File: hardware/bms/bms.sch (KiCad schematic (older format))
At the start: 199 parts, among them J1 Conn_01x08, J10 Conn_01x02, J11 Conn_01x02, J12 Conn_01x02, J13 Conn_01x10, J14 Conn_01x02, J15 Conn_01x02, J16 Cell Bypass, J2 Conn_01x04, J3 USB_B_Micro, J4 Conn_01x05, J5 Conn_01x04, J6 Conn_01x04, J7 Conn_01x03, J8 Conn_01x03, J9 Conn_01x02, M1 MountingHole, M2 MountingHole, M3 MountingHole, M4 MountingHole, M5 MountingHole, M6 MountingHole, Q1 BC817, Q10 ZXMP4A16G, Q11 IRF540N, Q12 IRF540N, Q13 BSS138, Q14 IRF540N, Q15 BSS138, Q16 BSS138, Q2 ZXMP4A16G, Q3 BSS138, Q4 BS170, Q5 IRF9540N, Q6 BC847, Q7 IRF9540N, Q8 BSS138, Q9 ZXMP4A16G, SW1 SW_DIP_x03, U1 USBLC6-2SC6, U2 STM32F042C6Tx, U3 TPS560430x3F, U4 TCAN334, U5 MAX485E, U6 LM5164DDAR, U7 LSI94202, Y1 8MHz

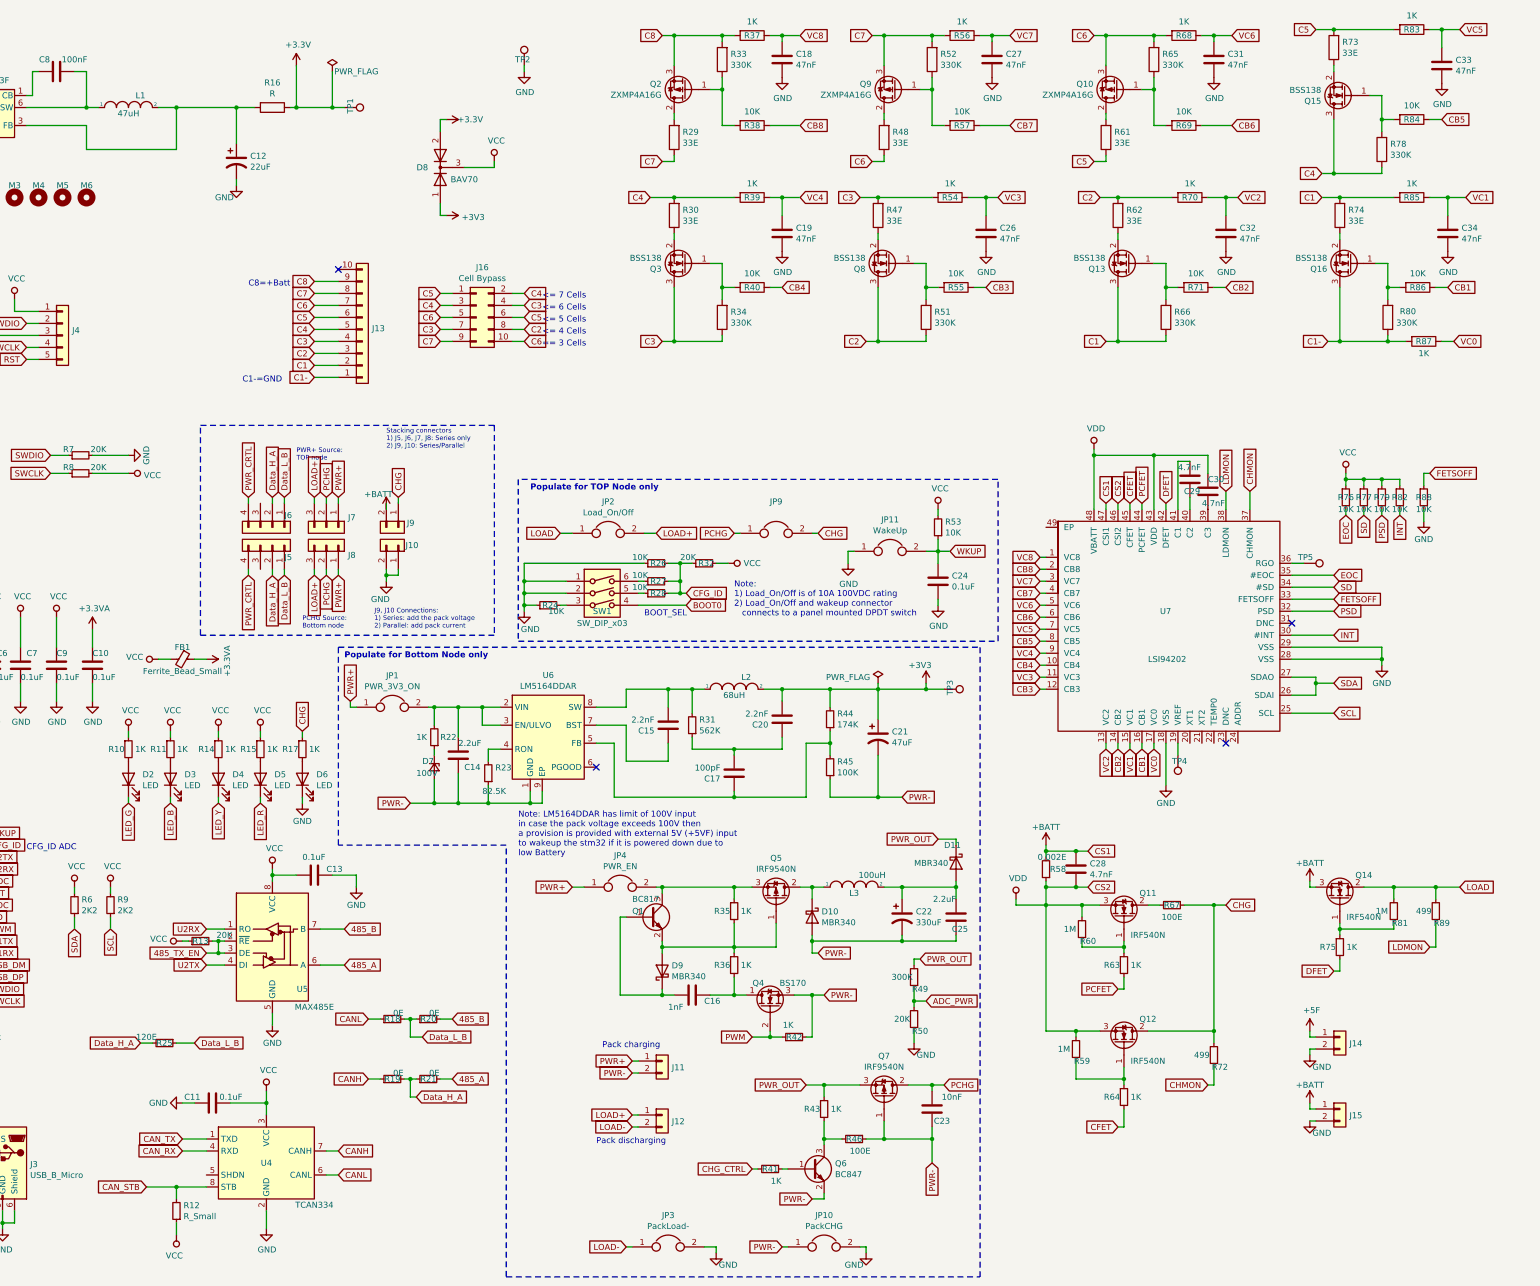
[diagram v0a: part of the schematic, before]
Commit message: created netlist
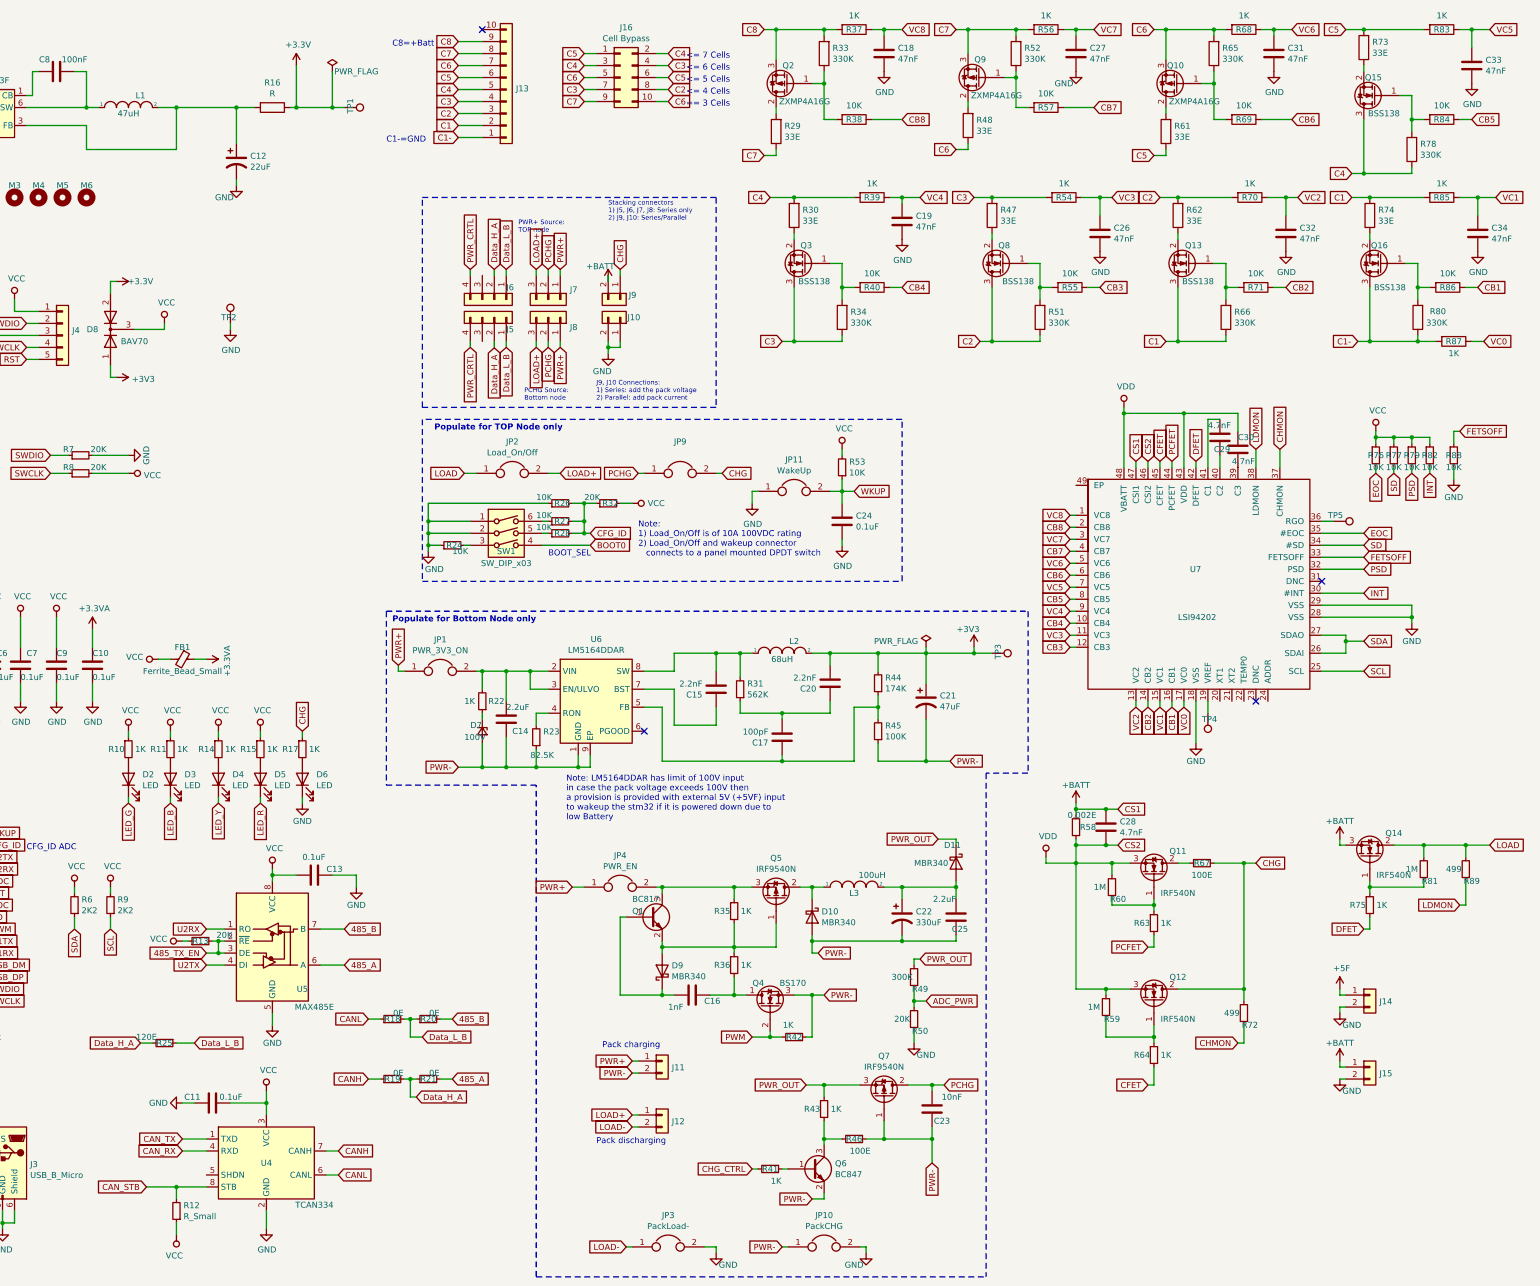
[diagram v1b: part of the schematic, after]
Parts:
- U1: footprint TO_SOT_Packages_SMD:SOT-23-6 -> Package_SO:TSOP-6_1.65x3.05mm_P0.95mm
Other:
- moved on the sheet: C14, C15, C17, C18, C19, C20, C21, C24, C26, C27, C28, C29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
